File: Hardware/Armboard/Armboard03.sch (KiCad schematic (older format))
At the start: 8 parts

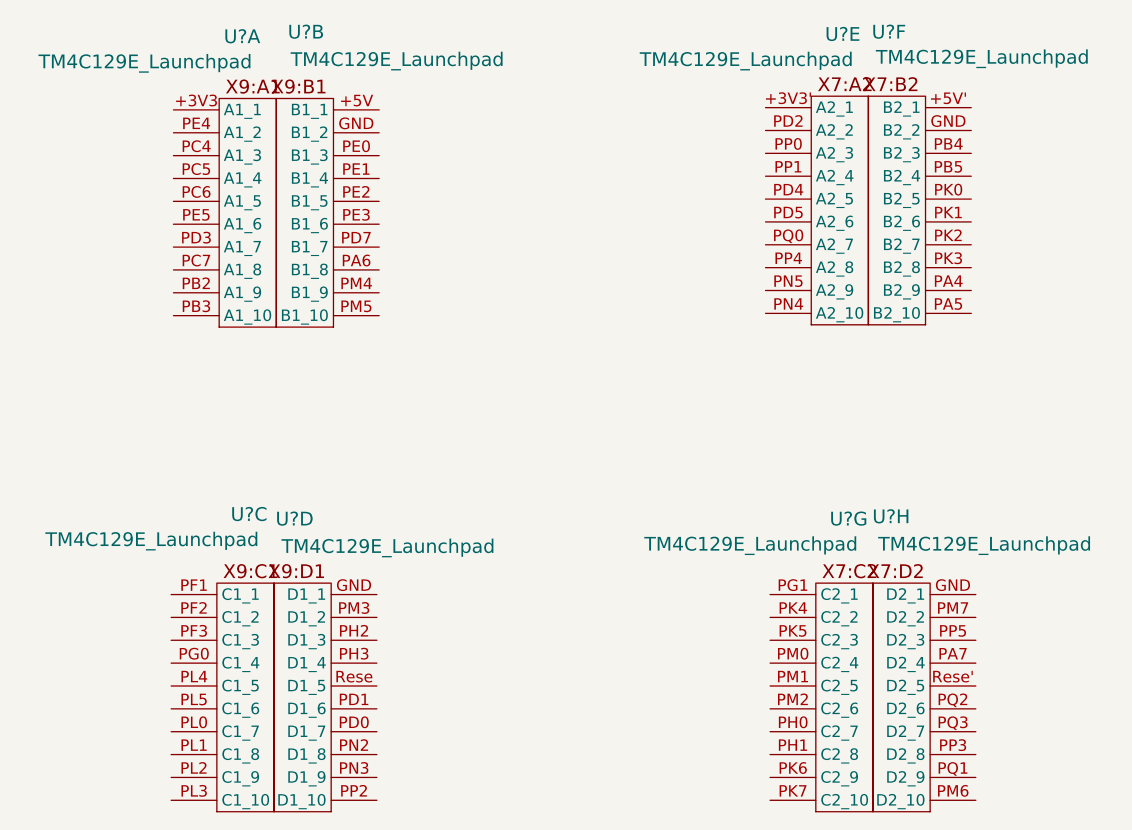
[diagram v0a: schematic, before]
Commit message: Tiva Updates
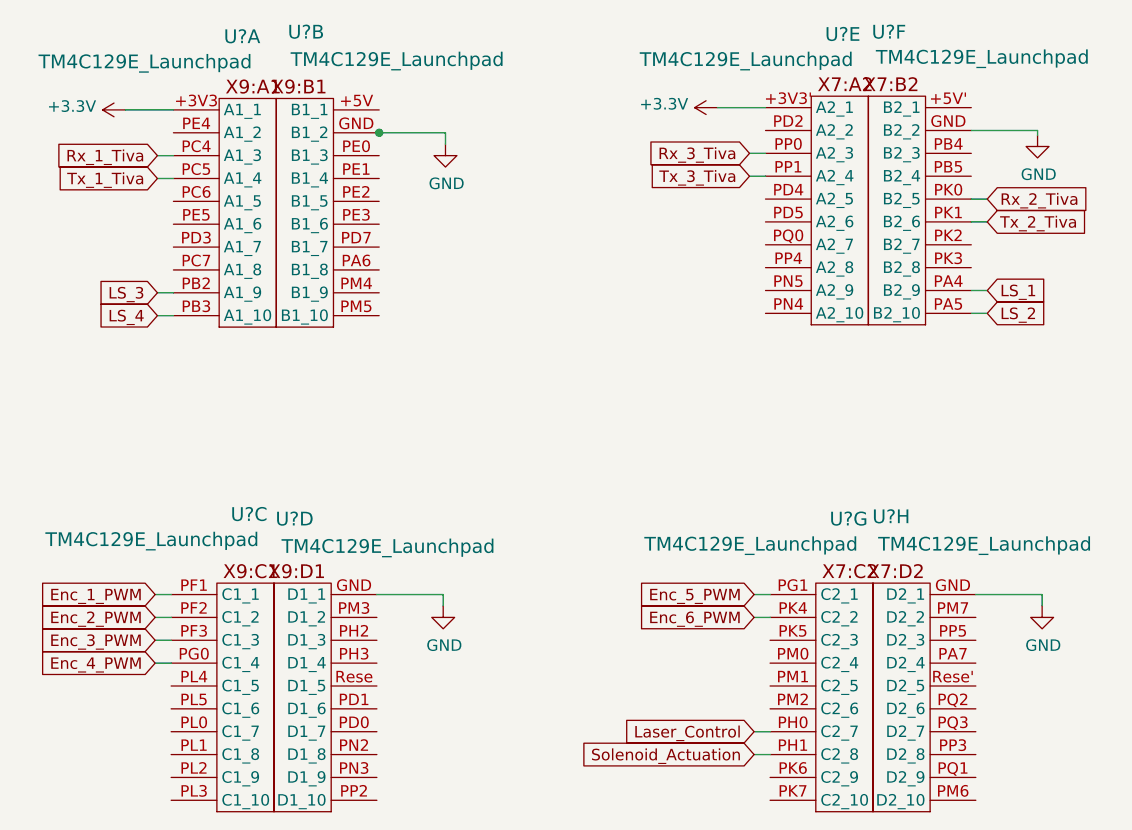
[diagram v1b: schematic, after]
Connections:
- net +3V3: now reaches U?.+3V3 (A1_1)
- net +3V3: now also U?.+3V3' (A2_1)
- net LS_3: now reaches U?.PB2 (A1_9)
- net LS_4: now reaches U?.PB3 (A1_10)
- net Rx_1_Tiva: now reaches U?.PC4 (A1_3)
- net Tx_1_Tiva: now reaches U?.PC5 (A1_4)
- net GND: now reaches U?.GND (B1_2)
- net GND: now also U?.GND (B2_2), U?.GND (D1_1), U?.GND (D2_1)
- net Enc_1_PWM: now reaches U?.PF1 (C1_1)
- net Enc_2_PWM: now reaches U?.PF2 (C1_2)
- net Enc_3_PWM: now reaches U?.PF3 (C1_3)
- net Enc_4_PWM: now reaches U?.PG0 (C1_4)
- net Rx_3_Tiva: now reaches U?.PP0 (A2_3)
- net Tx_3_Tiva: now reaches U?.PP1 (A2_4)
- net LS_1: now reaches U?.PA4 (B2_9)
- net LS_2: now reaches U?.PA5 (B2_10)
- net Rx_2_Tiva: now reaches U?.PK0 (B2_5)
- net Tx_2_Tiva: now reaches U?.PK1 (B2_6)
- net Enc_5_PWM: now reaches U?.PG1 (C2_1)
- net Laser_Control: now reaches U?.PH0 (C2_7)
- net Solenoid_Actuation: now reaches U?.PH1 (C2_8)
- net Enc_6_PWM: now reaches U?.PK4 (C2_2)
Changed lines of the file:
@@
 	-1   0    0    -1
 $EndComp
+$Comp
+L power:GND #PWR?
+U 1 1 5F83BEC8
+P 4800 2600
+F 0 "#PWR?" H 4800 2350 50  0001 C CNN
+F 1 "GND" H 4805 2427 50  0000 C CNN
+F 2 "" H 4800 2600 50  0001 C CNN
+F 3 "" H 4800 2600 50  0001 C CNN
+	1    4800 2600
+	1    0    0    -1
+$EndComp
+Wire Wire Line
+	4500 2550 4510 2550
+Wire Wire Line
+	4800 2550 4800 2600
+Connection ~ 4510 2550
+Wire Wire Line
+	4510 2550 4800 2550
+$Comp
+L power:+3.3V #PWR?
+U 1 1 5F83D247
+P 3400 2450
+F 0 "#PWR?" H 3400 2300 50  0001 C CNN
+F 1 "+3.3V" V 3415 2578 50  0000 L CNN
+F 2 "" H 3400 2450 50  0001 C CNN
+F 3 "" H 3400 2450 50  0001 C CNN
+	1    3400 2450
+	0    -1   -1   0
+$EndComp
+Wire Wire Line
+	3400 2450 3610 2450
+$Comp
+L power:+3.3V #PWR?
+U 1 1 5F83FA68
+P 5990 2440
+F 0 "#PWR?" H 5990 2290 50  0001 C CNN
+F 1 "+3.3V" V 6005 2568 50  0000 L CNN
+F 2 "" H 5990 2440 50  0001 C CNN
+F 3 "" H 5990 2440 50  0001 C CNN
+	1    5990 2440
+	0    -1   -1   0
+$EndComp
+Wire Wire Line
+	5990 2440 6200 2440
+$Comp
+L power:GND #PWR?
+U 1 1 5F83FD93
+P 7390 2560
+F 0 "#PWR?" H 7390 2310 50  0001 C CNN
+F 1 "GND" H 7395 2387 50  0000 C CNN
+F 2 "" H 7390 2560 50  0001 C CNN
+F 3 "" H 7390 2560 50  0001 C CNN
+	1    7390 2560
+	1    0    0    -1
+$EndComp
+$Comp
+L power:GND #PWR?
+U 1 1 5F83FFBB
+P 4790 4620
+F 0 "#PWR?" H 4790 4370 50  0001 C CNN
+F 1 "GND" H 4795 4447 50  0000 C CNN
+F 2 "" H 4790 4620 50  0001 C CNN
+F 3 "" H 4790 4620 50  0001 C CNN
+	1    4790 4620
+	1    0    0    -1
+$EndComp
+Wire Wire Line
+	4790 4570 4790 4620
+Wire Wire Line
+	4500 4570 4790 4570
+$Comp
+L power:GND #PWR?
+U 1 1 5F8401EF
+P 7410 4620
+F 0 "#PWR?" H 7410 4370 50  0001 C CNN
+F 1 "GND" H 7415 4447 50  0000 C CNN
+F 2 "" H 7410 4620 50  0001 C CNN
+F 3 "" H 7410 4620 50  0001 C CNN
+	1    7410 4620
+	1    0    0    -1
+$EndComp
+Wire Wire Line
+	7410 4570 7410 4620
+Wire Wire Line
+	7120 4570 7410 4570
+Text GLabel 3530 4570 0    50   Input ~ 0
+Enc_1_PWM
+Wire Wire Line
+	3600 4570 3530 4570
+Text GLabel 3530 4670 0    50   Input ~ 0
+Enc_2_PWM
+Wire Wire Line
+	3600 4670 3530 4670
+Text GLabel 3530 4770 0    50   Input ~ 0
+Enc_3_PWM
+Wire Wire Line
+	3600 4770 3530 4770
+Text GLabel 3530 4870 0    50   Input ~ 0
+Enc_4_PWM
+Wire Wire Line
+	3600 4870 3530 4870
+Text GLabel 6150 4570 0    50   Input ~ 0
+Enc_5_PWM
+Wire Wire Line
+	6220 4570 6150 4570
+Text GLabel 6150 4670 0    50   Input ~ 0
+Enc_6_PWM
+Wire Wire Line
+	6220 4670 6150 4670
+Text GLabel 7170 3340 2    50   Input ~ 0
+LS_2
+Wire Wire Line
+	7100 3340 7170 3340
+Text GLabel 7170 3240 2    50   Input ~ 0
+LS_1
+Wire Wire Line
+	7100 3240 7170 3240
+Text GLabel 3540 3250 0    50   Input ~ 0
+LS_3
+Wire Wire Line
+	3610 3250 3540 3250
+Text GLabel 3540 3350 0    50   Input ~ 0
+LS_4
+Wire Wire Line
+	3610 3350 3540 3350
+Text GLabel 6150 5170 0    50   Input ~ 0
+Laser_Control
+Wire Wire Line
+	6220 5170 6150 5170
+Text GLabel 6150 5270 0    50   Input ~ 0
+Solenoid_Actuation
+Wire Wire Line
+	6220 5270 6150 5270
+Text GLabel 3540 2650 0    50   Input ~ 0
+Rx_1_Tiva
+Wire Wire Line
+	3610 2650 3540 2650
+Text GLabel 3540 2750 0    50   Input ~ 0
+Tx_1_Tiva
+Wire Wire Line
+	3610 2750 3540 2750
+Text GLabel 7170 2940 2    50   Input ~ 0
+Tx_2_Tiva
+Wire Wire Line
+	7100 2940 7170 2940
+Text GLabel 7170 2840 2    50   Input ~ 0
+Rx_2_Tiva
+Wire Wire Line
+	7100 2840 7170 2840
+Wire Wire Line
+	7100 2540 7390 2540
+Wire Wire Line
+	7390 2540 7390 2560
+Text GLabel 6130 2640 0    50   Input ~ 0
+Rx_3_Tiva
+Wire Wire Line
+	6200 2640 6130 2640
+Text GLabel 6130 2740 0    50   Input ~ 0
+Tx_3_Tiva
+Wire Wire Line
+	6200 2740 6130 2740
 $EndSCHEMATC
